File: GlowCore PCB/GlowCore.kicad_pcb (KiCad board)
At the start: 4 copper layers, 20 x 38 mm, 59 parts, among them P1 Solder_Pad, P10 Solder_Pad, P11 Solder_Pad, P12 Solder_Pad, P13 Solder_Pad, P14 Solder_Pad, P15 Solder_Pad, P16 Solder_Pad, P17 Solder_Pad, P18 Solder_Pad, P19 Solder_Pad, P2 Solder_Pad, P20 Solder_Pad, P21 Solder_Pad, P22 Solder_Pad, P23 Solder_Pad, P24 Solder_Pad, P3 Solder_Pad, P4 Solder_Pad, P5 Solder_Pad, P6 Solder_Pad, P7 Solder_Pad, P8 Solder_Pad, P9 Solder_Pad, SW1 TS24CA, SW2 TS24CA, SW3 TS24CA, U1 SN74LVC1G373DBVR, U10 AP40P05, U11 74LVC2G04DW-7, U2 AP40P05, U3 ESP32-S3-MINI-1-N8, U4 AP40P05, U5 AO3400A, U6 SN74LVC2T45DCUR, U7 SPX3819M5-L-3-3_TR, U8 SK9822-EC20, U9 AP40P05

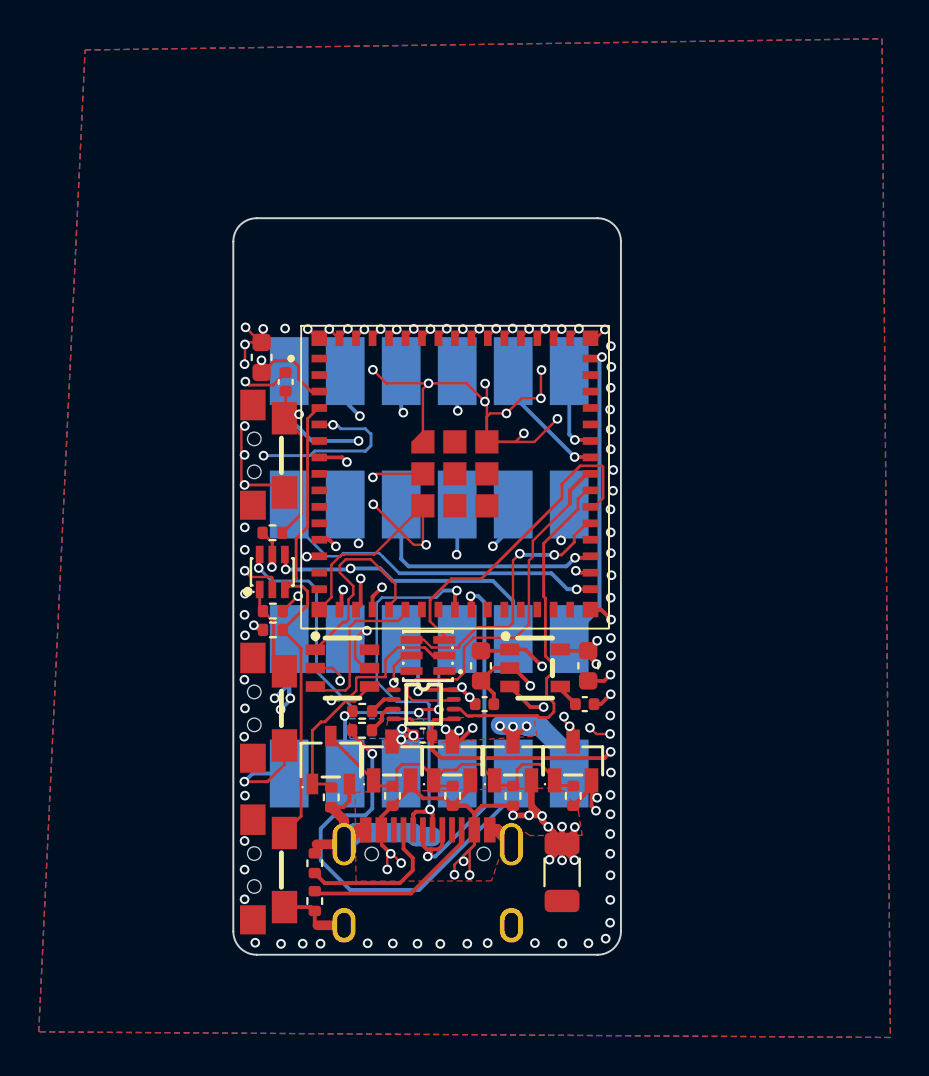
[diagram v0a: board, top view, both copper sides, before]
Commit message: updated pcb design
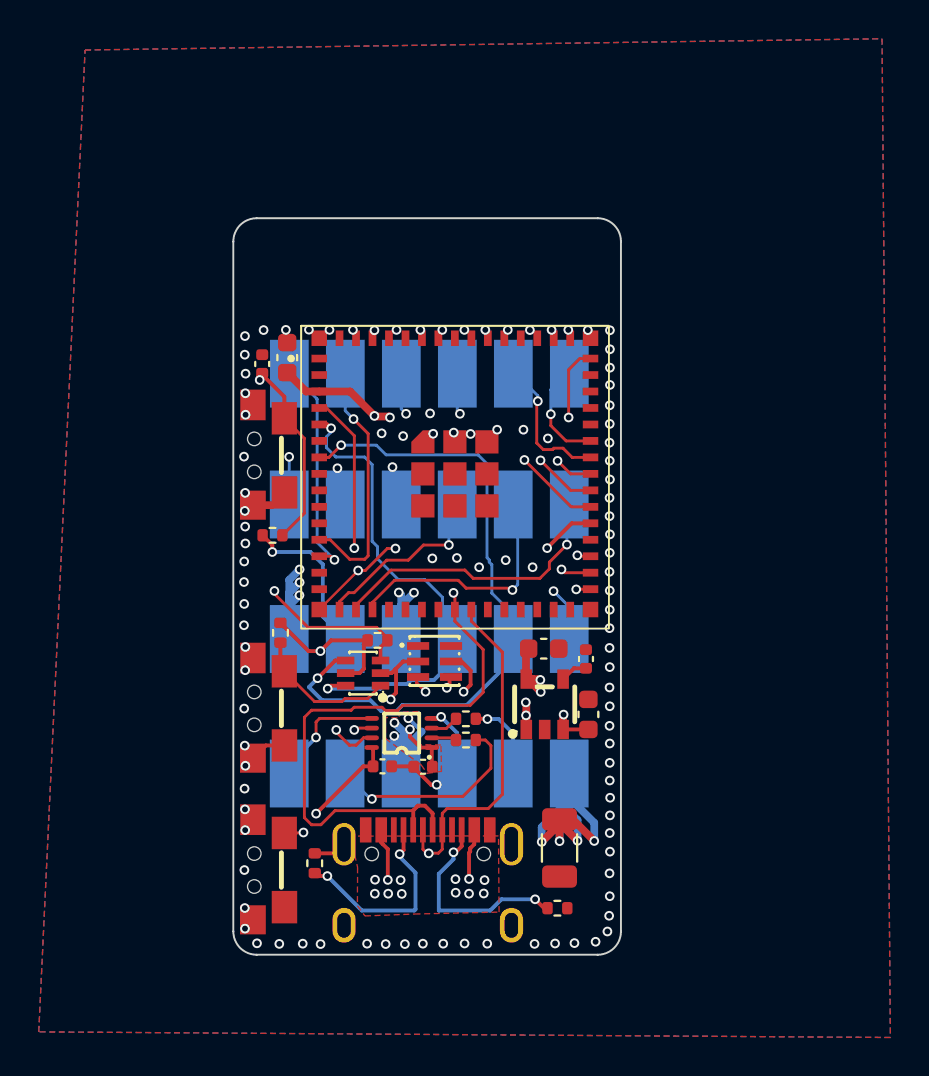
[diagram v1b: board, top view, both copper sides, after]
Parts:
- removed R13, R14, R3, R4, R5: 100K, Resistor_SMD:R_0402_1005Metric
- removed U10, U2, U4, U9: AP40P05, footprint:SOT-23-3_L2.9-W1.3-P1.90-LS2.4-BR
- removed U5: AO3400A, footprint:SOT-23-3_L2.9-W1.6-P1.90-LS2.8-BR
- removed U8: SK9822-EC20, footprint:LED-SMD_6P-L2.0-W2.0-P0.80-TL
- U1: value SN74LVC1G373DBVR -> SK9822-EC20; footprint footprint:SOT-23-6_L2.9-W1.6-P0.95-LS2.8-BR -> footprint:LED-SMD_6P-L2.0-W2.0-P0.80-TL
- U3: value ESP32-S3-MINI-1-N8 -> ESP32-S3-MINI-1-N4R2
- moved R7 12.5 mm to (165.3, 98.9), turned to 180 degrees
- moved U11 7.01 mm to (155.3, 86.8), turned to 0 degrees
- moved C5 6.17 mm to (156.3, 91.6)
- moved C6 6.08 mm to (166.9, 88.9), turned to -90 degrees
- moved R10 5.55 mm to (160.6, 90.3), turned to 0 degrees
- moved R2 5.43 mm to (156.0, 85.1)
- moved R11 5.39 mm to (160.6, 89.2), turned to 0 degrees
- moved U1 4.76 mm to (159.0, 86.2), turned to 0 degrees
- moved C8 2.46 mm to (164.6, 85.5), turned to 180 degrees
- moved C7 2.33 mm to (166.8, 86.1), turned to -90 degrees
- moved U7 1.93 mm to (164.7, 88.4), turned to -90 degrees
- moved U6 1.88 mm to (157.3, 89.9), turned to 0 degrees
- moved C4 1.61 mm to (158.4, 91.6), turned to 180 degrees
- moved C3 1.52 mm to (150.1, 70.8)
- moved C2 1.32 mm to (151.4, 70.5)
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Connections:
- C4 pad 1: 5V AFTER MOSFET -> VBUS
- C5 pad 1: 3.3V AFTER MOSFET -> +3V3
- P1 pad 1: 5V AFTER MOSFET -> VBUS
- P18 pad 1: 3.3V AFTER MOSFET -> +3V3
- P4 pad 1: 5V AFTER MOSFET -> VBUS
- SW1 pad 1: unconnected-(SW1-Pad1) -> GND
- SW1 pad 2: unconnected-(SW1-Pad2) -> GND
- SW2 pad 1: unconnected-(SW2-Pad1) -> GND
- SW2 pad 2: unconnected-(SW2-Pad2) -> GND
- SW3 pad 1: unconnected-(SW3-Pad1) -> GND
- SW3 pad 2: unconnected-(SW3-Pad2) -> GND
- U1 pad 1: IO15/LED LETCH EN -> unconnected-(U1-SDO-Pad1)
- U1 pad 3: IO16/POWERMOSFETS -> IO40/STATUS LED DATA
- U1 pad 4: Net-(U1-Q) -> IO39/STATUS LED CLOCK
- U1 pad 5: +3V3 -> VBUS
- U3 pad 19: IO15/LED LETCH EN -> unconnected-(U3-IO15-Pad19)
- U3 pad 20: IO16/POWERMOSFETS -> unconnected-(U3-IO16-Pad20)
- U6 pad 1: 5V AFTER MOSFET -> VBUS
- U6 pad 8: 3.3V AFTER MOSFET -> +3V3
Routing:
- net GND: track 128.9 -> 27.4 mm, vias 100 -> 109
- net +3V3: track 27.3 -> 84.0 mm
- net 5V AFTER MOSFET: track 22.0 -> 0.00 mm, vias 10 -> 0
- net Net-(U10-G): track 18.9 -> 0.00 mm
- net LED2 DATA OUT: track 22.9 -> 5.47 mm
- net IO20/USB D+: track 43.3 -> 60.2 mm, vias 3 -> 2
- net IO9/I2C SCL: track 25.3 -> 11.6 mm, vias 2 -> 1
- net IO3/ACTIONBUTTON: track 22.3 -> 35.0 mm, vias 3 -> 2
- net IO0/BOOT: track 25.2 -> 36.5 mm, vias 0 -> 3
- net IO15/LED LETCH EN: track 10.5 -> 0.00 mm
- net IO1/POWERBUTTON: track 35.0 -> 25.7 mm, vias 5 -> 2
- net 3.3V AFTER MOSFET: track 9.05 -> 0.00 mm, vias 5 -> 0
- net IO42/LED1: track 20.5 -> 29.3 mm, vias 0 -> 2
- net IO16/POWERMOSFETS: track 8.37 -> 0.00 mm
- net IO41/LED2: track 18.5 -> 26.6 mm, vias 0 -> 2
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- added copper zone on In2.Cu, net VBUS
- removed copper zone on In1.Cu, net +3V3
- removed copper zone on In1.Cu, net 3.3V AFTER MOSFET
- removed copper zone on B.Cu, net 5V AFTER MOSFET
- removed copper zone on F.Cu, net 5V AFTER MOSFET
- removed copper zone on In1.Cu, net 5V AFTER MOSFET
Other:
- board text removed: "O"
